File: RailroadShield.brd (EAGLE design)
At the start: 99.6 x 78.7 mm, 70 parts, among them J1 5520250-3, J2 5520250-3, J3 5520250-3, J4 5520426-4, J5 5520426-4, J6 KK-156-5, J7 KK-156-5, J8 MSTB-02, Q1 PMBT2222, U1 LM393M, U2 MCP2515-ST, U3 MCP2551-SN, U4 MAX3468CSA, U5 MAX3468CSA, U6 MAX3468CSA, U7 LM317LCDR, U8 6N137SD, Y1 16Mhz

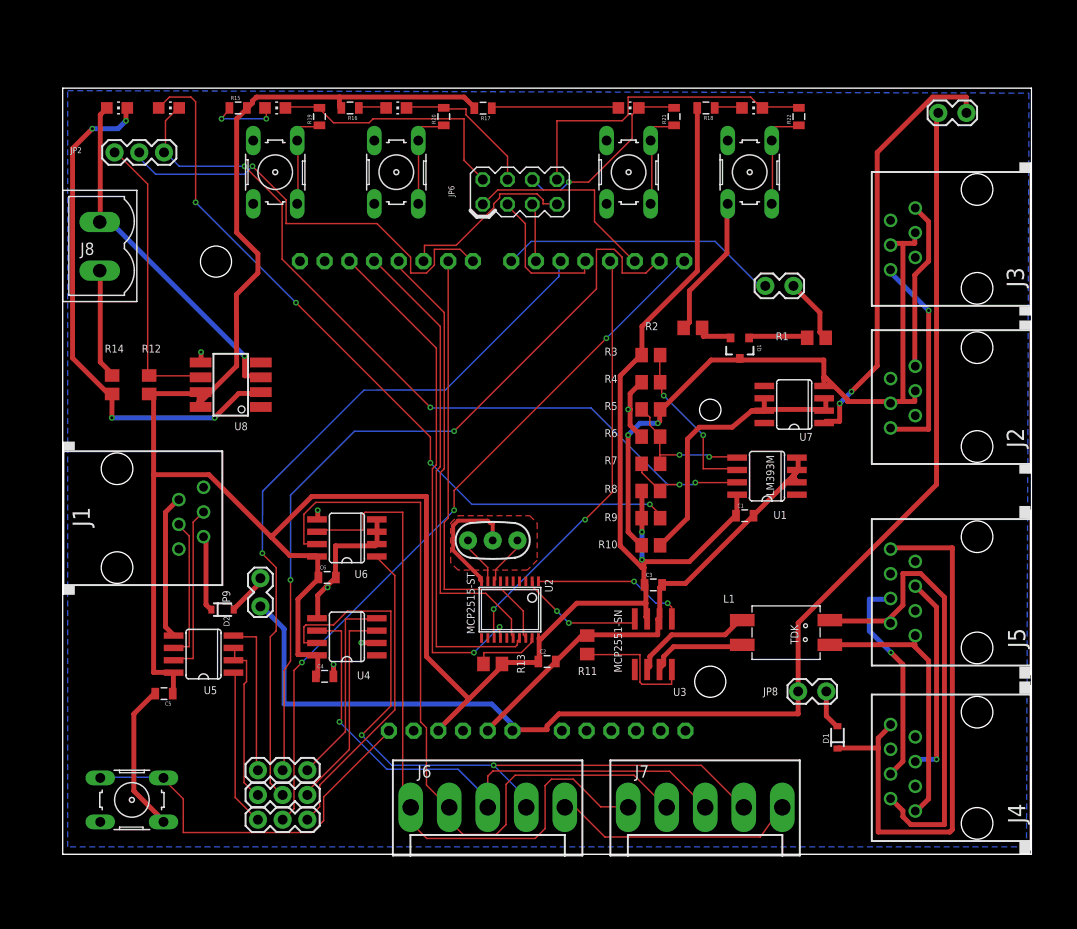
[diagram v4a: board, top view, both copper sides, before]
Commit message: 2.3
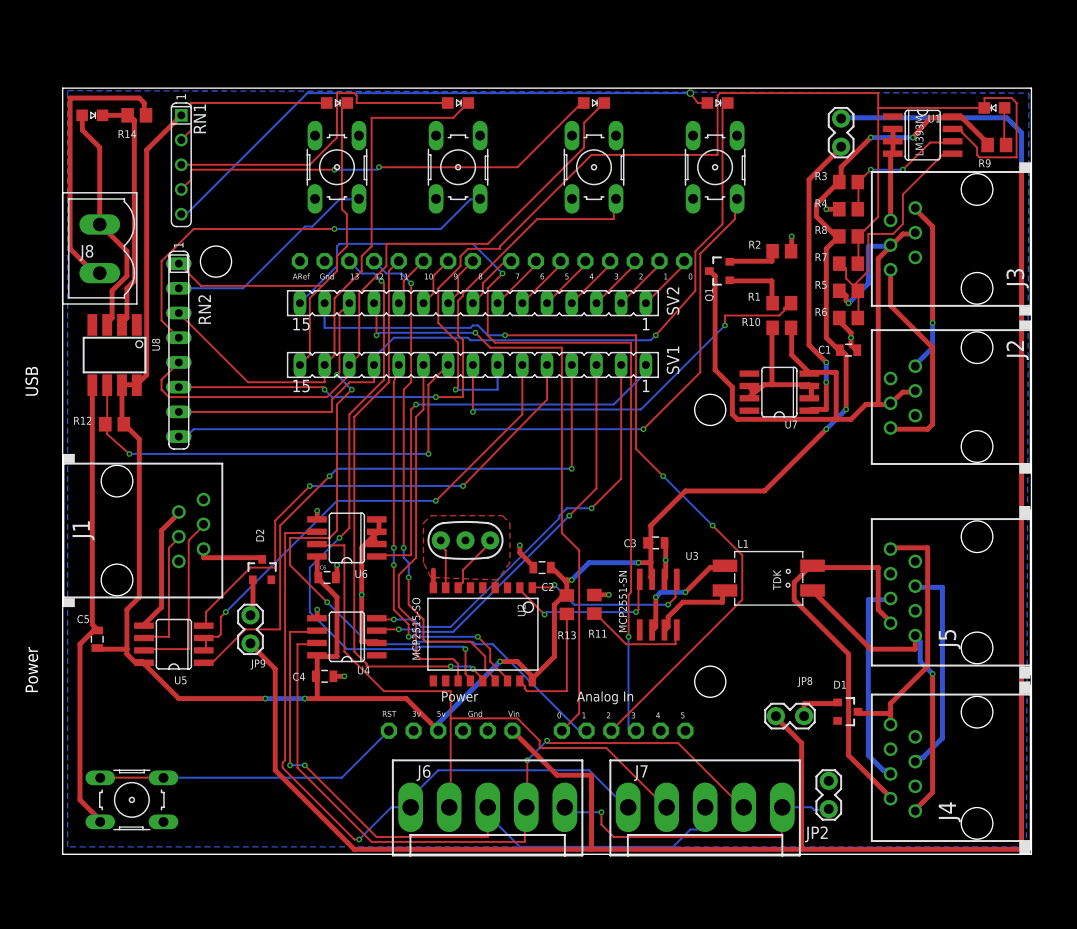
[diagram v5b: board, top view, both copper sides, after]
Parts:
- removed JP3: RxD, MCP:1X03
- removed JP4: EN, MCP:1X03
- removed JP5: TxD, MCP:1X03
- removed JP6: MA04-2, MCP:MA04-2
- removed JP7: LNTX, MCP:1X02_LOCK
- removed R15, R16, R17, R18, R19, R20, R21, R22: 660R, MCP:0805
- added RN1: 660R, resistor-sil:SIL5
- added RN2: 660R, resistor-sil:SIL8
- added SV1, SV2: (no value), con-lsta:FE15
- D1, D2: device MCP:SOD-323 -> MCP:SOT23-3
- JP2: value RXD-LN -> ShieldGnd; device MCP:1X03 -> MCP:1X02_LOCK
- U2: value MCP2515-ST -> MCP2515-SO; device MCP:TSSOP20 -> MCP:SO-18W
- moved JP2 97.9 mm to (78.7, 7.37), turned to 270 degrees
- moved LED6 84.8 mm to (95.8, 76.7), turned to 90 degrees
- moved R9 52.3 mm to (96.0, 72.9)
- moved U1 38.5 mm to (88.4, 73.9), turned to 270 degrees
- moved R8 33.1 mm to (80.8, 63.5)
- moved R7 28.9 mm to (80.8, 60.7), turned to 0 degrees
- moved R14 27.8 mm to (7.62, 75.9), turned to 180 degrees
- moved R3 27.0 mm to (80.8, 69.1)
- moved R4 27.0 mm to (80.8, 66.3)
- moved R10 26.1 mm to (73.9, 54.1), turned to 0 degrees
- moved R5 23.7 mm to (80.8, 57.9), turned to 0 degrees
- moved R6 23.7 mm to (80.8, 55.1)
- moved C1 20.1 mm to (80.8, 51.8)
- moved JP1 13.1 mm to (80.0, 72.9), turned to 90 degrees
- moved U8 12.3 mm to (5.33, 51.3), turned to 180 degrees
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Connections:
- removed net D11: U$1.D11, U2.16
- removed net D12: U$1.D12, U2.17
- removed net D13: U$1.D13, U2.14
- removed net S1+: R19.1, S1.3, S1.4
- removed net S2+: R20.1, S2.3, S2.4
- removed net S3+: R21.1, S3.3, S3.4
- removed net S4+: R22.1, S4.3, S4.4
- new net A0: SV2.12, U$1.A0
- new net A1: SV2.13, U$1.A1
- new net A2: SV2.14, U$1.A2
- new net A3: SV2.15, U$1.A3
- new net CANCS: SV1.11, U2.16
- new net CANINT: SV1.10, U2.12
- new net MISO: U$1.D12, U2.15
- new net MOSI: U$1.D11, U2.14
- new net N$16: RN2.2, S1.3
- new net N$17: RN2.4, S2.3
- new net N$18: RN2.6, S3.3
- new net N$19: RN2.8, S4.3
- new net SCK: U$1.D13, U2.13
- net /RESET: now also U2.17; no longer U2.19
- net CAN-PWR+: now also D1.3; no longer D1.1
- net CMRIRX: now also SV1.1; no longer JP3.1
- net CMRITX: now also SV1.2; no longer JP5.1
- net CMRITXEN: now also SV1.3; no longer JP4.1
- net D0: now also SV2.1; no longer JP3.2
- net D1: now also SV2.2; no longer JP5.2
- net D10: now also SV2.11; no longer JP6.7
- net D2: now also SV2.3; no longer JP6.1
- net D3: now also SV2.4; no longer U2.13
- net D4: now also SV2.5; no longer JP6.3
- net D5: now also SV2.6; no longer JP4.2
- net D6: now also SV2.7; no longer JP6.5
- net D7: now also SV2.8; no longer JP7.2
- net D8: now also SV2.9; no longer JP2.2
- net D9: now also SV2.10; no longer U2.18
- net DCCRX: now also SV1.9; no longer JP2.1
- net GND: now also JP2.1, U2.9; no longer S1.2, S2.2, S3.2, S4.2, U2.10
- net IO1: now also RN2.1, SV1.15; no longer JP6.2, R19.2
- net IO2: now also RN2.3, SV1.14; no longer JP6.4, R20.2
- net IO3: now also RN2.5, SV1.13; no longer JP6.6, R21.2
- net IO4: now also RN2.7, SV1.12; no longer JP6.8, R22.2
- net LNRX: now also SV1.7; no longer JP2.3
- net LNTX: now also SV1.8; no longer JP7.1
- net N$12: now also U2.8; no longer U2.9
- net N$13: now also U2.7; no longer U2.8
- net N$14: now also D2.1; no longer D2.2
- net N$15: now also D1.1; no longer D1.2
- net N$2: now also LED1.A, RN1.2; no longer LED2.A, R16.1
- net N$3: now also LED2.A, RN1.3; no longer LED3.A, R17.1
- net N$4: now also LED3.A, RN1.4; no longer LED4.A, R18.1
- net N$5: now also LED4.A, RN1.5; no longer LED1.A, R15.1
- net N$6: now also JP2.2
- net NCE-PWR+: now also D2.3; no longer D2.1
- net NCERX: now also SV1.4; no longer JP3.3
- net NCETX: now also SV1.5; no longer JP5.3
- net NCETXEN: now also SV1.6; no longer JP4.3
- net VCC: now also RN1.1, U2.18; no longer R15.2, R16.2, R17.2, R18.2, U2.20
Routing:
- net A3: track 0.00 -> 88.6 mm, vias 0 -> 2
- net A2: track 0.00 -> 85.8 mm, vias 0 -> 3
- net V+: track 134.2 -> 219.6 mm, vias 0 -> 1
- net N$19: track 0.00 -> 75.8 mm, vias 0 -> 1
- net D1: track 81.8 -> 6.02 mm, vias 2 -> 0
- net L6+: track 77.8 -> 4.03 mm, vias 4 -> 0
- net A1: track 0.00 -> 70.8 mm, vias 0 -> 3
- net D0: track 74.6 -> 6.02 mm, vias 3 -> 0
- net D5: track 73.9 -> 6.02 mm, vias 1 -> 0
- net A0: track 0.00 -> 64.0 mm, vias 0 -> 2
- net SCK: track 0.00 -> 62.7 mm, vias 0 -> 3
- net N$18: track 0.00 -> 61.8 mm, vias 0 -> 2
- net MOSI: track 0.00 -> 56.8 mm, vias 0 -> 2
- net D13: track 53.3 -> 0.00 mm, vias 2 -> 0
- net MISO: track 0.00 -> 52.5 mm, vias 0 -> 3
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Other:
- board text added: "/CS"
- board text added: "/INT"
- board text added: "2011.07"
- board text added: "A0"
- board text added: "A1"
- board text added: "A2"
- board text added: "A3"
- board text added: "BlueIO"
- board text added: "Buttons/LEDs"
- board text added: "D3"
- board text added: "D9"
- board text added: "GoldIO"
- board text added: "Loconet Termination"
- board text added: "Made in the PCR, Coast Division, NMRA"
- board text added: "RX"
- board text added: "Rev. 2.3"
- board text added: "TX"
- board text added: "TX-EN"
- board text added: "X"
- board text added: "XpressNet"
- board text added: "Y"
- board text added: "seeed: 31126"
- board text added: "xIO"
- board text added: "yIO"
- board text removed: "1"
- board text removed: "2"
- board text removed: "2010.10"
- board text removed: "3"
- board text removed: "4"
- board text removed: "Loconet Termination Power"
- board text removed: "Rev. 2.2"
